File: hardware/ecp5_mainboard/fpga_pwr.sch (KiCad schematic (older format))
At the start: 62 parts, among them U11 ECP5UM5G_85_CABGA756

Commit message: hardware/mainboard: Assign some footprints
Signed-off-by: David Shah <dave@ds0.me>
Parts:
- C31, C33, C34, C83, C84: footprint (none) -> Capacitor_SMD:C_1210_3225Metric
- C32, C35, C36, C37, C80, C81, C85: footprint (none) -> Capacitor_SMD:C_0603_1608Metric
- C38, C39, C40, C41, C42, C43, C44, C45, C46, C47, C48, C49, C50, C51, C52, C53, C54, C55, C56, C57, C58, C59, C60, C61, C62, C63, C64, C65, C66, C67, C68, C69, C70, C71, C72, C73, C74, C75, C76, C77, C78, C79, C82: footprint (none) -> Capacitor_SMD:C_0402_1005Metric
- C86: footprint (none) -> Capacitor_SMD:C_1206_3216Metric
- L10, L11, L7, L8, L9: footprint (none) -> Inductor_SMD:L_0603_1608Metric

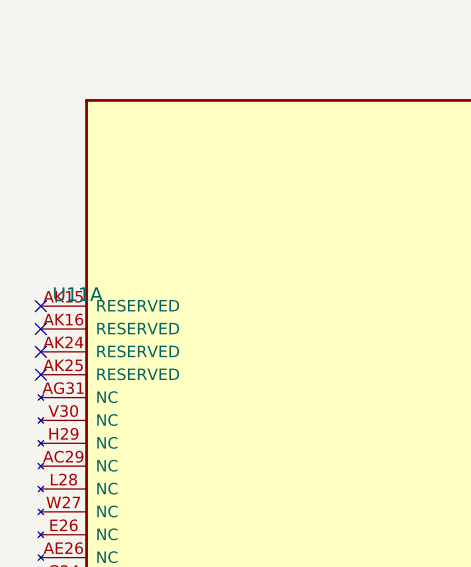
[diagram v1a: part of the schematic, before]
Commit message: hardware/mainboard: Assign more footprints
Signed-off-by: David Shah <dave@ds0.me>
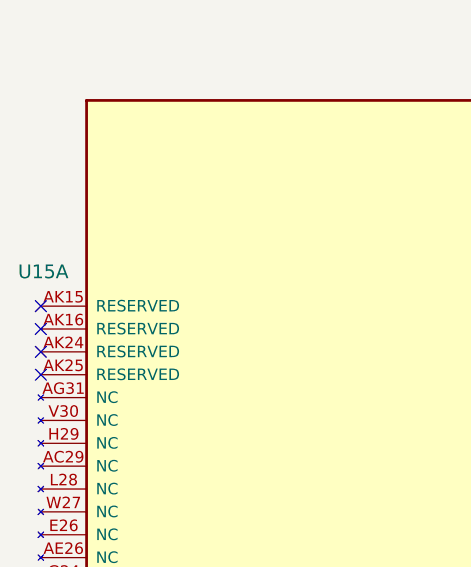
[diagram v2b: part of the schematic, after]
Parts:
- U15: renamed from U11; footprint (none) -> Custom Parts:CABGA756_27x27mm_p0.8mm
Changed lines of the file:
@@
 $EndDescr
 $Comp
-L ECP5UM5G:ECP5UM5G_85_CABGA756 U11
+L ECP5UM5G:ECP5UM5G_85_CABGA756 U15
 U 1 1 5B5F6062
 P 4900 13150
-F 0 "U11" H 4950 13200 60  0000 L CNN
+F 0 "U15" H 4800 13300 60  0000 L CNN
 F 1 "ECP5UM5G_85_CABGA756" H 28331 11497 60  0000 L CNN
-F 2 "" H 4900 13150 50  0001 C CNN
+F 2 "Custom Parts:CABGA756_27x27mm_p0.8mm" H 4900 13150 50  0001 C CNN
 F 3 "" H 4900 13150 50  0001 C CNN
 F 4 "ECP5UM5G_85" H 5050 13100 60  0001 R CNN "manf#"

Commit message: hardware/mainboard: Place FPGA decoupling
Signed-off-by: David Shah <dave@ds0.me>
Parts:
- C42, C43, C46, C47, C49, C50, C59, C60, C62, C63, C65, C66: footprint Capacitor_SMD:C_0402_1005Metric -> Capacitor_SMD:C_0201_0603Metric
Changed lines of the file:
@@
 F 0 "C66" H 21592 10946 50  0000 L CNN
 F 1 "10n" H 21592 10855 50  0000 L CNN
-F 2 "Capacitor_SMD:C_0402_1005Metric" H 21500 10900 50  0001 C CNN
+F 2 "Capacitor_SMD:C_0201_0603Metric" H 21500 10900 50  0001 C CNN
 F 3 "~" H 21500 10900 50  0001 C CNN
 	1    21500 10900
@@
 F 0 "C63" H 21292 10946 50  0000 L CNN
 F 1 "10n" H 21292 10855 50  0000 L CNN
-F 2 "Capacitor_SMD:C_0402_1005Metric" H 21200 10900 50  0001 C CNN
+F 2 "Capacitor_SMD:C_0201_0603Metric" H 21200 10900 50  0001 C CNN
 F 3 "~" H 21200 10900 50  0001 C CNN
 	1    21200 10900
@@
 F 0 "C60" H 20992 10946 50  0000 L CNN
 F 1 "1n" H 20992 10855 50  0000 L CNN
-F 2 "Capacitor_SMD:C_0402_1005Metric" H 20900 10900 50  0001 C CNN
+F 2 "Capacitor_SMD:C_0201_0603Metric" H 20900 10900 50  0001 C CNN
 F 3 "~" H 20900 10900 50  0001 C CNN
 	1    20900 10900
@@
 F 0 "C65" H 21592 10346 50  0000 L CNN
 F 1 "10n" H 21592 10255 50  0000 L CNN
-F 2 "Capacitor_SMD:C_0402_1005Metric" H 21500 10300 50  0001 C CNN
+F 2 "Capacitor_SMD:C_0201_0603Metric" H 21500 10300 50  0001 C CNN
 F 3 "~" H 21500 10300 50  0001 C CNN
 	1    21500 10300
@@
 F 0 "C62" H 21292 10346 50  0000 L CNN
 F 1 "10n" H 21292 10255 50  0000 L CNN
-F 2 "Capacitor_SMD:C_0402_1005Metric" H 21200 10300 50  0001 C CNN
+F 2 "Capacitor_SMD:C_0201_0603Metric" H 21200 10300 50  0001 C CNN
 F 3 "~" H 21200 10300 50  0001 C CNN
 	1    21200 10300
@@
 F 0 "C59" H 20992 10346 50  0000 L CNN
 F 1 "1n" H 20992 10255 50  0000 L CNN
-F 2 "Capacitor_SMD:C_0402_1005Metric" H 20900 10300 50  0001 C CNN
+F 2 "Capacitor_SMD:C_0201_0603Metric" H 20900 10300 50  0001 C CNN
 F 3 "~" H 20900 10300 50  0001 C CNN
 	1    20900 10300
@@
 F 0 "C46" H 12842 11246 50  0000 L CNN
 F 1 "10n" H 12842 11155 50  0000 L CNN
-F 2 "Capacitor_SMD:C_0402_1005Metric" H 12750 11200 50  0001 C CNN
+F 2 "Capacitor_SMD:C_0201_0603Metric" H 12750 11200 50  0001 C CNN
 F 3 "~" H 12750 11200 50  0001 C CNN
 	1    12750 11200
@@
 F 0 "C49" H 13142 11246 50  0000 L CNN
 F 1 "1n" H 13142 11155 50  0000 L CNN
-F 2 "Capacitor_SMD:C_0402_1005Metric" H 13050 11200 50  0001 C CNN
+F 2 "Capacitor_SMD:C_0201_0603Metric" H 13050 11200 50  0001 C CNN
 F 3 "~" H 13050 11200 50  0001 C CNN
 	1    13050 11200
@@
 F 0 "C47" H 12842 11696 50  0000 L CNN
 F 1 "10n" H 12842 11605 50  0000 L CNN
-F 2 "Capacitor_SMD:C_0402_1005Metric" H 12750 11650 50  0001 C CNN
+F 2 "Capacitor_SMD:C_0201_0603Metric" H 12750 11650 50  0001 C CNN
 F 3 "~" H 12750 11650 50  0001 C CNN
 	1    12750 11650
@@
 F 0 "C50" H 13142 11696 50  0000 L CNN
 F 1 "1n" H 13142 11605 50  0000 L CNN
-F 2 "Capacitor_SMD:C_0402_1005Metric" H 13050 11650 50  0001 C CNN
+F 2 "Capacitor_SMD:C_0201_0603Metric" H 13050 11650 50  0001 C CNN
 F 3 "~" H 13050 11650 50  0001 C CNN
 	1    13050 11650
@@
 F 0 "C42" H 12242 10546 50  0000 L CNN
 F 1 "10n" H 12242 10455 50  0000 L CNN
-F 2 "Capacitor_SMD:C_0402_1005Metric" H 12150 10500 50  0001 C CNN
+F 2 "Capacitor_SMD:C_0201_0603Metric" H 12150 10500 50  0001 C CNN
 F 3 "~" H 12150 10500 50  0001 C CNN
 	1    12150 10500
@@
 F 0 "C43" H 12242 11046 50  0000 L CNN
 F 1 "10n" H 12242 10955 50  0000 L CNN
-F 2 "Capacitor_SMD:C_0402_1005Metric" H 12150 11000 50  0001 C CNN
+F 2 "Capacitor_SMD:C_0201_0603Metric" H 12150 11000 50  0001 C CNN
 F 3 "~" H 12150 11000 50  0001 C CNN
 	1    12150 11000

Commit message: hardware/mainboard: BoM fixes, add USB power option
Signed-off-by: David Shah <dave@ds0.me>
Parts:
- C86: footprint Capacitor_SMD:C_1206_3216Metric -> Capacitor_SMD:C_1210_3225Metric
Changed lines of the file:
@@
 EESchema Schematic File Version 4
 LIBS:ecp5_mainboard-cache
-EELAYER 26 0
+EELAYER 29 0
 EELAYER END
 $Descr A1 33110 23386
@@
 F 0 "C86" H 23842 11596 50  0000 L CNN
 F 1 "47µ" H 23842 11505 50  0000 L CNN
-F 2 "Capacitor_SMD:C_1206_3216Metric" H 23750 11550 50  0001 C CNN
+F 2 "Capacitor_SMD:C_1210_3225Metric" H 23750 11550 50  0001 C CNN
 F 3 "~" H 23750 11550 50  0001 C CNN
 	1    23750 11550
